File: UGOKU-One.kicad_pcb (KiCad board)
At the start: 2 copper layers, 63 x 63 mm, 35 parts, among them CN1 Conn_01x04, CN2 Conn_01x04, CN3 Conn_01x04, J2 Conn_02x03_Odd_Even, J3 Conn_01x02_Male, J4 PA10, P1 USB_C_Plug_USB2.0, Q1 2SC2712, SW1 PF1, SW2 RESET, SW3 SW_Push_DPDT, SW5 SW_Push_DPDT, T3 PTS_1.5_2, T5 MultiBoardMini_Libraries:PTS_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, U1 K7803-500R3, U3 TB67H450FNG_EL, U7 ESP32-WROOM-32, U8 TB67H450FNG_EL

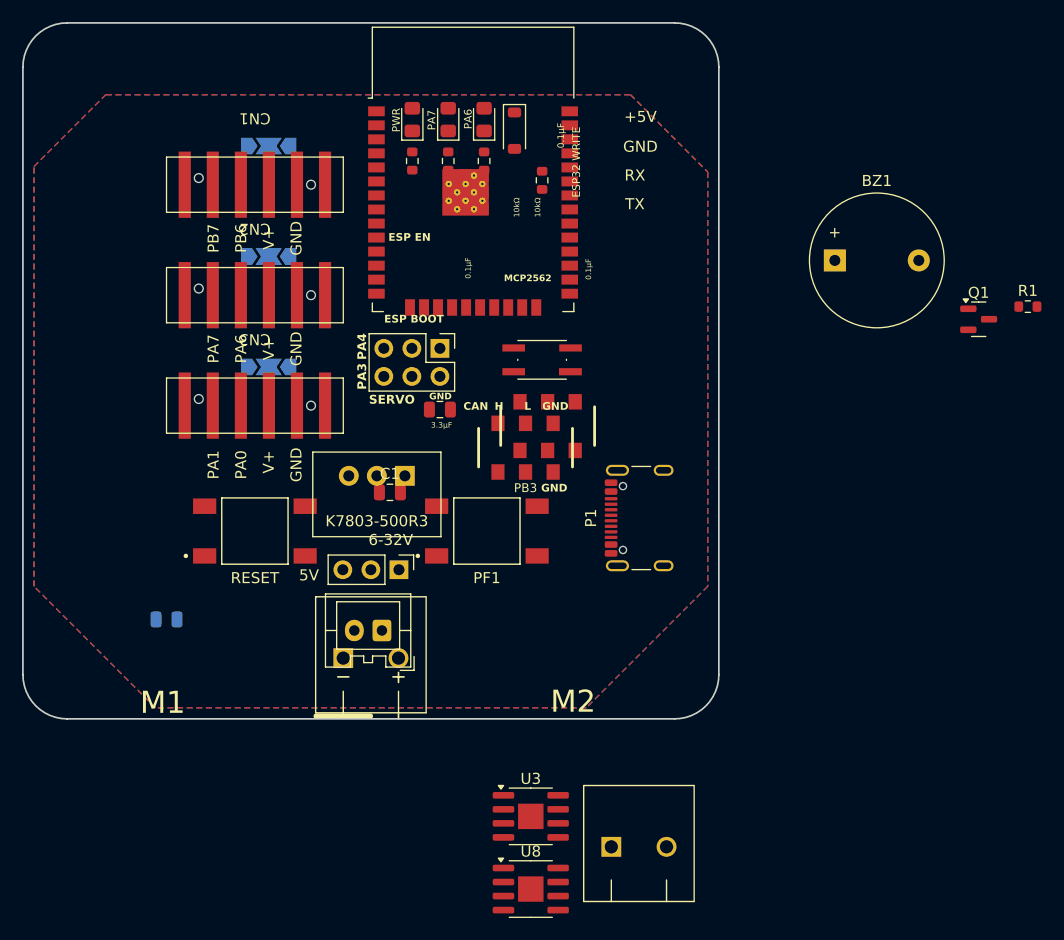
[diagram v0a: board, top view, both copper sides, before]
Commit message: make concept
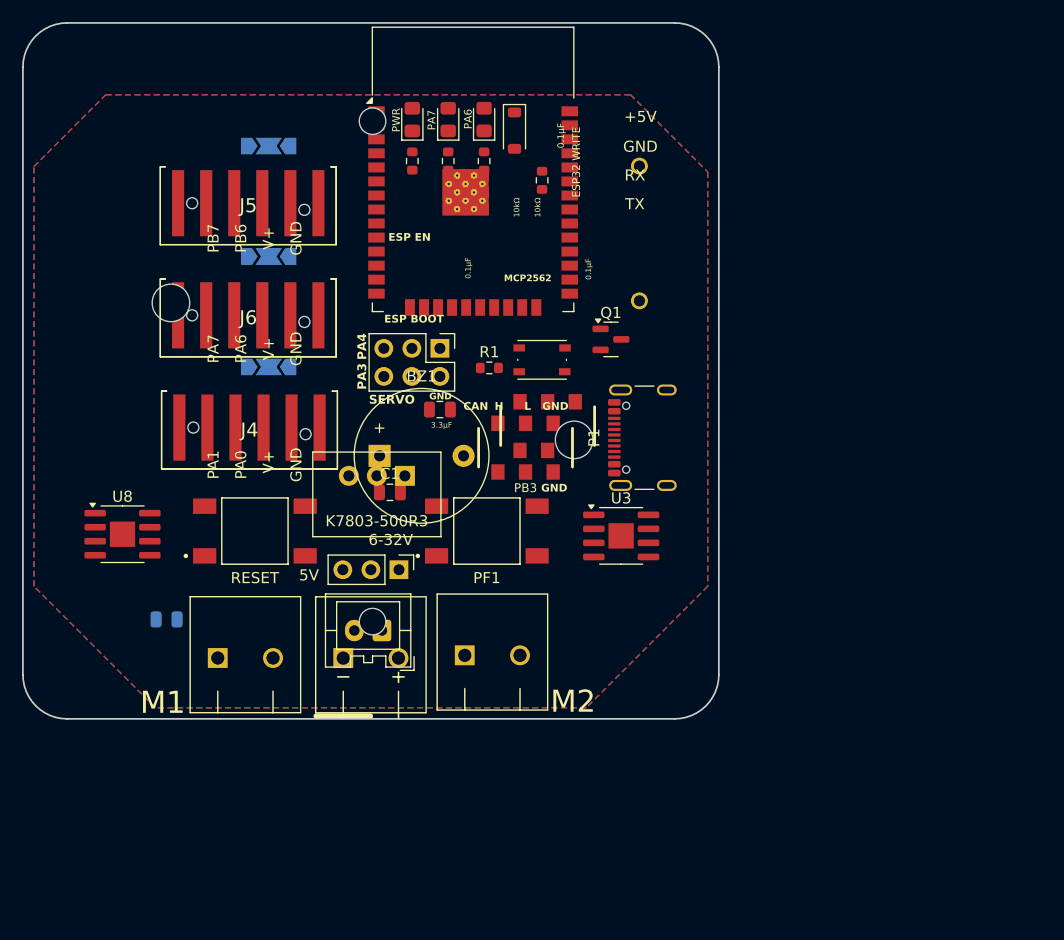
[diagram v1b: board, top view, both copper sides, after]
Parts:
- removed CN1, CN2, CN3: Conn_01x04, UGOKU-One_Libraries:har-flexicon_2.54_4pin
- added BT1: Battery, 0_UGOKU-One_Lib:BAT_2481, B.Cu at (0.15, 0.05)
- added J4: 14110413001000, 0_UGOKU-One_Lib:14110413001000, F.Cu at (-11.0, 5.13)
- added J5: 14110413001000, 0_UGOKU-One_Lib:14110413001000, F.Cu at (-11.1, -15.2)
- added J6: 14110413001000, 0_UGOKU-One_Lib:14110413001000, F.Cu at (-11.1, -5.03)
- added T4: PTS_1.5_2, 0_UGOKU-One_Lib:PTS_1.5_2, F.Cu at (11.0, 25.8)
- T5: footprint UGOKU-One_Libraries:PTS_1.5_2 -> 0_UGOKU-One_Lib:PTS_1.5_2
- moved R1 49.1 mm to (10.7, -0.27)
- moved U8 49.0 mm to (-22.5, 14.8)
- moved BZ1 44.8 mm to (0.79, 7.69)
- moved T5 39.5 mm to (-11.4, 26.0)
- moved Q1 33.3 mm to (21.7, -2.85)
- moved U3 26.7 mm to (22.7, 14.9)
- moved P1 7.28 mm to (25.7, 6.05)
